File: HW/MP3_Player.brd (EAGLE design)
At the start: 210 x 15 mm, 81 parts, among them J2 LIPO-BATTERY-CONNECTOR, J3 USD-SDIO-SOCKETJLH, Q1 8MHz, Q2 12.288MHz, U1 3.3V/150mA, U2 1.8V/100mA, U4 VS1053B, U5 MCP73831

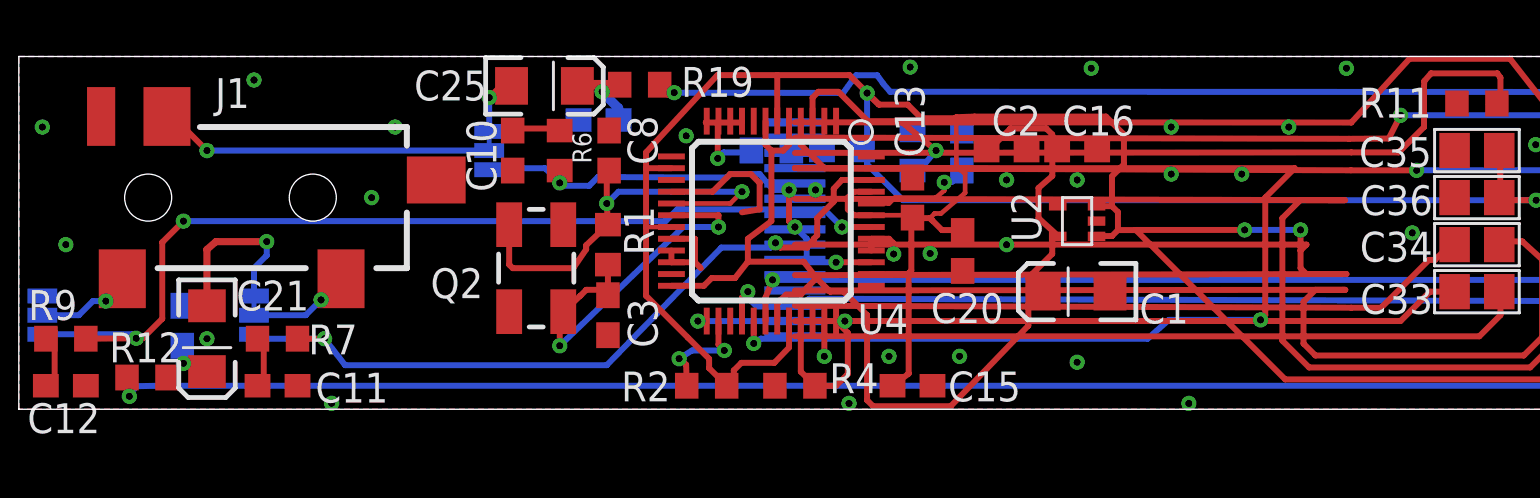
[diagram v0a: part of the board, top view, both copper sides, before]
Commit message: changed OLED footprint
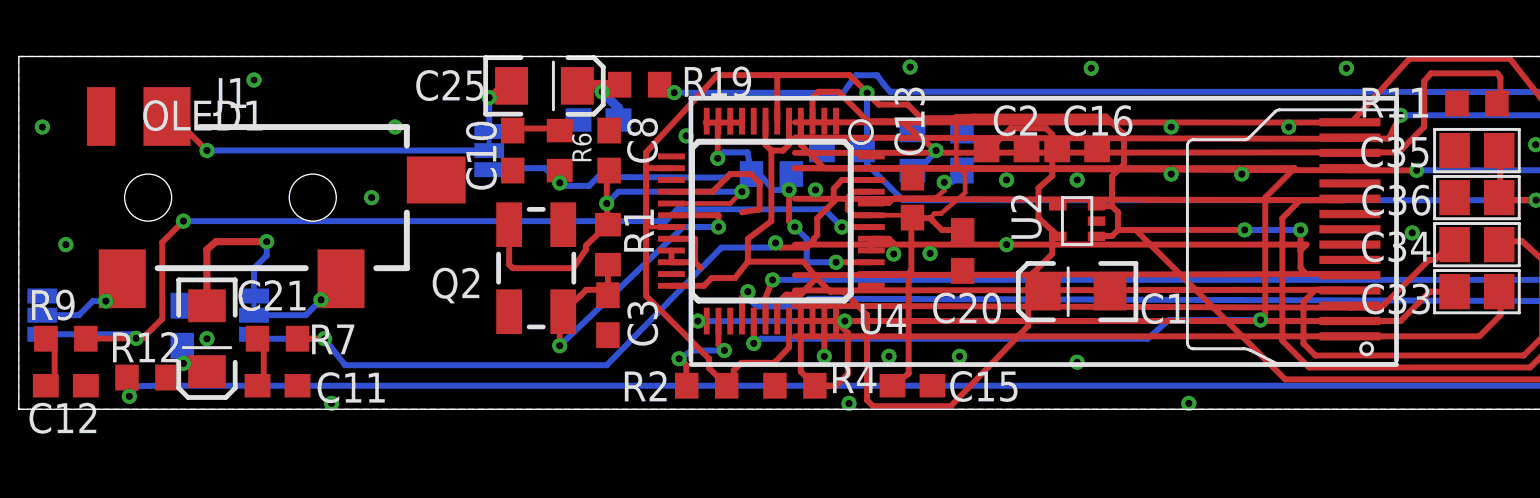
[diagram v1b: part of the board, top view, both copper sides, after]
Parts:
- moved OLED1 8.00 mm to (40.8, 7.65), flipped to the top
- moved R3 1.00 mm to (32.0, 10.0)
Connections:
- net MP3-CS: now also U$3.20
- net MP3-DCS: now also U$3.21
- net MP3-DREQ: now also U$3.18
- net MP3-RST: now also U$3.19
- net OLED-RST: now also U$3.25
- net PWM_L: now also U$3.30
- net PWM_R: now also U$3.29
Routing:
- net G1: track 4.86 -> 5.62 mm
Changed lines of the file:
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@@
 <layer number="20" name="Dimension" color="15" fill="1" visible="yes" active="yes"/>
 <layer number="21" name="tPlace" color="7" fill="1" visible="yes" active="yes"/>
-<layer number="22" name="bPlace" color="7" fill="1" visible="yes" active="yes"/>
+<layer number="22" name="bPlace" color="7" fill="1" visible="no" active="yes"/>
 <layer number="23" name="tOrigins" color="15" fill="1" visible="yes" active="yes"/>
-<layer number="24" name="bOrigins" color="15" fill="1" visible="yes" active="yes"/>
+<layer number="24" name="bOrigins" color="15" fill="1" visible="no" active="yes"/>
 <layer number="25" name="tNames" color="7" fill="1" visible="yes" active="yes"/>
 <layer number="26" name="bNames" color="7" fill="1" visible="no" active="yes"/>
-<layer number="27" name="tValues" color="7" fill="1" visible="no" active="yes"/>
+<layer number="27" name="tValues" color="7" fill="1" visible="yes" active="yes"/>
 <layer number="28" name="bValues" color="7" fill="1" visible="no" active="yes"/>
-<layer number="29" name="tStop" color="7" fill="3" visible="no" active="yes"/>
+<layer number="29" name="tStop" color="7" fill="3" visible="yes" active="yes"/>
 <layer number="30" name="bStop" color="7" fill="6" visible="no" active="yes"/>
-<layer number="31" name="tCream" color="7" fill="4" visible="yes" active="yes"/>
+<layer number="31" name="tCream" color="7" fill="4" visible="no" active="yes"/>
 <layer number="32" name="bCream" color="7" fill="5" visible="no" active="yes"/>
 <layer number="33" name="tFinish" color="6" fill="3" visible="no" active="yes"/>
@@
 <layer number="46" name="Milling" color="3" fill="1" visible="no" active="yes"/>
 <layer number="47" name="Measures" color="7" fill="1" visible="yes" active="yes"/>
-<layer number="48" name="Document" color="7" fill="1" visible="yes" active="yes"/>
+<layer number="48" name="Document" color="7" fill="1" visible="no" active="yes"/>
 <layer number="49" name="Reference" color="7" fill="1" visible="no" active="yes"/>
 <layer number="50" name="dxf" color="7" fill="1" visible="no" active="no"/>
-<layer number="51" name="tDocu" color="7" fill="1" visible="yes" active="yes"/>
-<layer number="52" name="bDocu" color="7" fill="1" visible="no" active="yes"/>
+<layer number="51" name="tDocu" color="7" fill="1" visible="no" active="yes"/>
+<layer number="52" name="bDocu" color="7" fill="1" visible="yes" active="yes"/>
 <layer number="53" name="tGND_GNDA" color="7" fill="9" visible="no" active="no"/>
 <layer number="54" name="bGND_GNDA" color="1" fill="9" visible="no" active="no"/>
@@
 <attribute name="VALUE" x="28.615" y="-0.905" size="1.27" layer="27"/>
 </element>
-<element name="R3" library="rcl" package="R0603" value="100k" x="32" y="11" smashed="yes" rot="MR0">
-<attribute name="NAME" x="31.785" y="11.835" size="1.27" layer="26" rot="MR0"/>
-<attribute name="VALUE" x="32.635" y="9.095" size="1.27" layer="28" rot="MR0"/>
+<element name="R3" library="rcl" package="R0603" value="100k" x="32" y="10" smashed="yes" rot="MR0">
+<attribute name="NAME" x="31.785" y="10.835" size="1.27" layer="26" rot="MR0"/>
+<attribute name="VALUE" x="32.635" y="8.095" size="1.27" layer="28" rot="MR0"/>
 </element>
 <element name="R4" library="rcl" package="R0603" value="100k" x="33" y="1" smashed="yes">
@@
 <attribute name="SUPPLIER-ID" value="SM02B-GHS-TB(LF)(SN)" x="189.049" y="9.954" size="1.778" layer="27" rot="R180" display="off"/>
 </element>
-<element name="OLED1" library="pero_library" package="UG-2832HSWEG04" value="UG-2832HSWEG04" x="48.8" y="7.652" smashed="yes" rot="MR0">
-<attribute name="NAME" x="84.4" y="11.852" size="1.27" layer="26" rot="MR0"/>
-<attribute name="VALUE" x="78.8" y="0.152" size="1.016" layer="28" rot="MR0"/>
+<element name="OLED1" library="pero_library" package="UG-2832HSWEG04" value="UG-2832HSWEG04" x="40.8" y="7.652" smashed="yes">
+<attribute name="NAME" x="5.2" y="11.852" size="1.27" layer="25"/>
+<attribute name="VALUE" x="10.8" y="0.152" size="1.016" layer="27"/>
 </element>
 <element name="C33" library="microbuilder" package="0805" value="1.0µF" x="62" y="5" smashed="yes">
@@
 <wire x1="61.05" y1="9" x2="61.05" y2="11" width="0" layer="19" extent="1-1"/>
 <wire x1="59.25" y1="7.5" x2="61.05" y2="9" width="0" layer="19" extent="1-1"/>
-<wire x1="33" y1="6.352" x2="59.25" y2="7.5" width="0" layer="19" extent="1-1"/>
+<wire x1="56.6" y1="6.352" x2="59.25" y2="7.5" width="0" layer="19" extent="1-1"/>
 <wire x1="56.45" y1="14.5" x2="61.15" y2="13" width="0" layer="19" extent="1-1"/>
 <wire x1="54" y1="12" x2="56.45" y2="14.5" width="0" layer="19" extent="1-1"/>
@@
 <wire x1="40" y1="2.25" x2="38.85" y2="1" width="0" layer="19" extent="1-1"/>
 <wire x1="38" y1="9.85" x2="37" y2="7.25" width="0" layer="19" extent="1-1"/>
-<wire x1="32.85" y1="11" x2="33.25" y2="11.25" width="0" layer="19" extent="1-16"/>
+<wire x1="32.85" y1="10" x2="33.25" y2="11.25" width="0" layer="19" extent="1-16"/>
 <wire x1="34.15" y1="11" x2="34.25" y2="10.25" width="0" layer="19" extent="1-16"/>
 <wire x1="33.875" y1="9.325" x2="34.25" y2="10.25" width="0" layer="19" extent="1-1"/>
 <wire x1="38" y1="11.85" x2="37.6" y2="10.25" width="0" layer="19" extent="1-16"/>
-<wire x1="31.5" y1="9.625" x2="32.85" y2="11" width="0" layer="19" extent="1-16"/>
+<wire x1="31.5" y1="9.625" x2="32.85" y2="10" width="0" layer="19" extent="1-16"/>
 <wire x1="27.75" y1="7.25" x2="27.75" y2="9.25" width="0" layer="19" extent="1-1"/>
 <wire x1="40.1" y1="11.85" x2="38" y2="11.85" width="0" layer="19" extent="16-16"/>
@@
 <wire x1="29.718" y1="10.668" x2="29.972" y2="10.922" width="0.254" layer="16"/>
 <wire x1="29.718" y1="12.192" x2="29.718" y2="10.668" width="0.254" layer="1"/>
-<wire x1="30.988" y1="10.922" x2="31.15" y2="11" width="0.254" layer="16"/>
+<wire x1="30.988" y1="10.922" x2="31.15" y2="10" width="0.254" layer="16"/>
 <wire x1="29.718" y1="12.192" x2="29.21" y2="12.192" width="0.254" layer="1"/>
 <wire x1="29.21" y1="12.192" x2="29.25" y2="12.25" width="0.254" layer="1"/>
@@
 <signal name="MP3-CS">
 <contactref element="U4" pad="23"/>
+<contactref element="U$3" pad="20"/>
+<wire x1="27.75" y1="5.75" x2="175.5" y2="9.4" width="0" layer="19" extent="1-1"/>
 </signal>
 <signal name="MP3-DCS">
 <contactref element="U4" pad="13"/>
+<contactref element="U$3" pad="21"/>
+<wire x1="27.75" y1="10.75" x2="175" y2="9.4" width="0" layer="19" extent="1-1"/>
 </signal>
 <signal name="MP3-RST">
@@
 <wire x1="36.1" y1="12.25" x2="37.5" y2="12.25" width="0.254" layer="1"/>
 <wire x1="37.5" y1="12.25" x2="39" y2="11" width="0.254" layer="1"/>
+<contactref element="U$3" pad="19"/>
+<wire x1="39" y1="11" x2="176" y2="9.4" width="0" layer="19" extent="1-1"/>
 </signal>
 <signal name="MP3-DREQ">
 <contactref element="U4" pad="8"/>
+<contactref element="U$3" pad="18"/>
+<wire x1="31.25" y1="12.25" x2="176.5" y2="9.4" width="0" layer="19" extent="1-1"/>
 </signal>
 <signal name="N$20">
@@
 <contactref element="OLED1" pad="8"/>
 <contactref element="U$3" pad="26"/>
-<wire x1="33" y1="7.652" x2="173.6" y2="7" width="0" layer="19" extent="1-1"/>
+<wire x1="56.6" y1="7.652" x2="173.6" y2="7" width="0" layer="19" extent="1-1"/>
 </signal>
 <signal name="OLED-RST">
 <contactref element="OLED1" pad="9"/>
+<contactref element="U$3" pad="25"/>
+<wire x1="56.6" y1="8.302" x2="173.6" y2="7.5" width="0" layer="19" extent="1-1"/>
 </signal>
 <signal name="OLED-DC">
@@
 <wire x1="27.866" y1="13.462" x2="27.588" y2="13.462" width="0.4064" layer="1"/>
 <wire x1="27.588" y1="13.462" x2="27.25" y2="13.8" width="0.4064" layer="1"/>
+<contactref element="U$3" pad="29"/>
+<wire x1="176.784" y1="5.842" x2="173.6" y2="5.5" width="0" layer="19" extent="1-16"/>
 </signal>
 <signal name="PWM_L">
@@
 <wire x1="6" y1="1" x2="174.228" y2="1" width="0.254" layer="16"/>
 <wire x1="174.228" y1="1" x2="176.276" y2="3.048" width="0.254" layer="16"/>
+<contactref element="U$3" pad="30"/>
+<wire x1="176.276" y1="3.048" x2="173.6" y2="5" width="0" layer="19" extent="1-16"/>
 </signal>
 <signal name="N$25">
